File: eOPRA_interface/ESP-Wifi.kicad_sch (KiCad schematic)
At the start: 18 parts, among them SW1 SW_Push

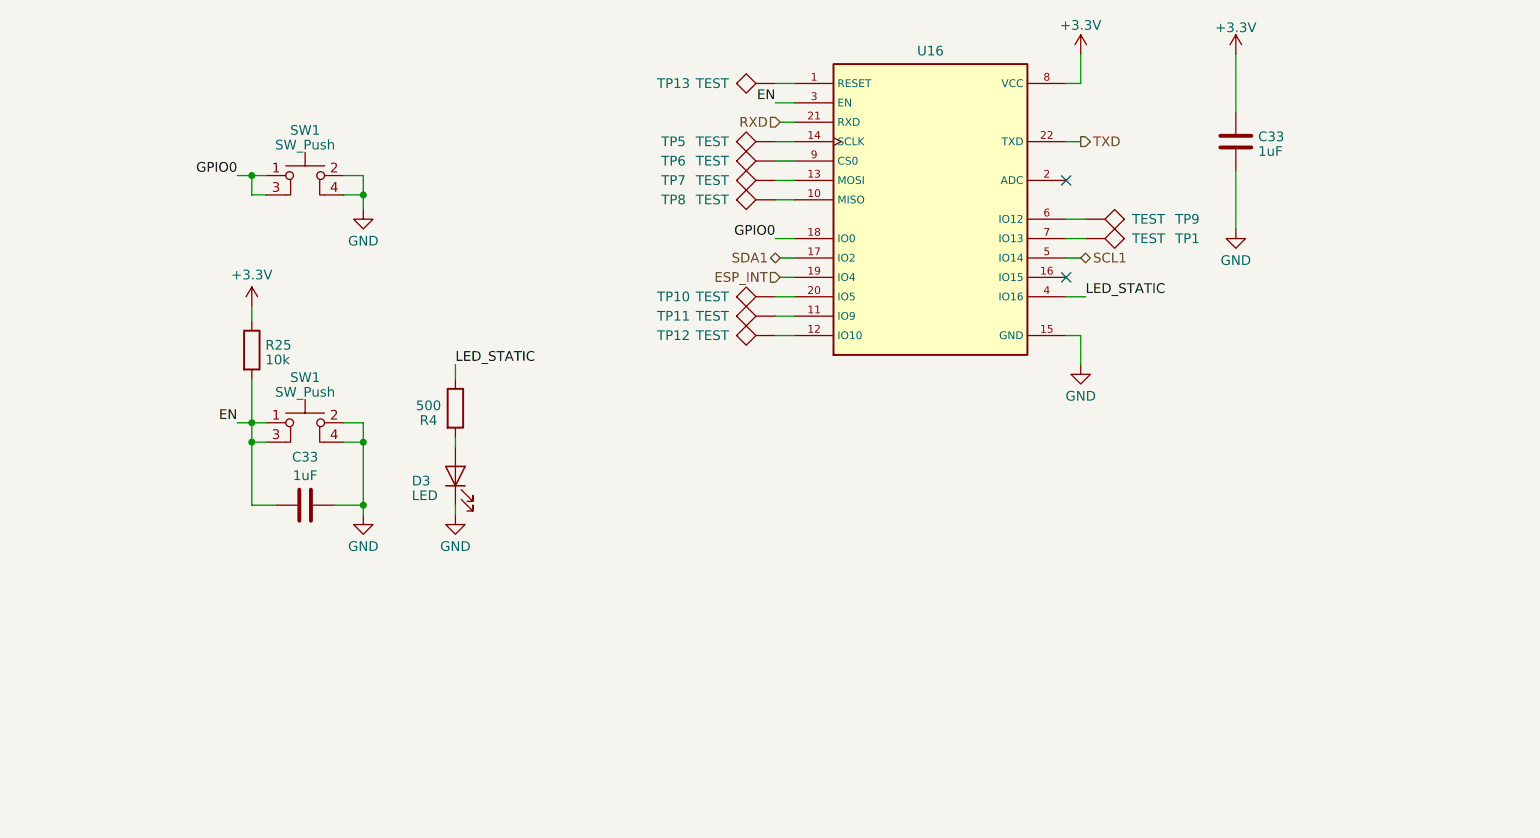
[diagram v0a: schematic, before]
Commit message: stuff
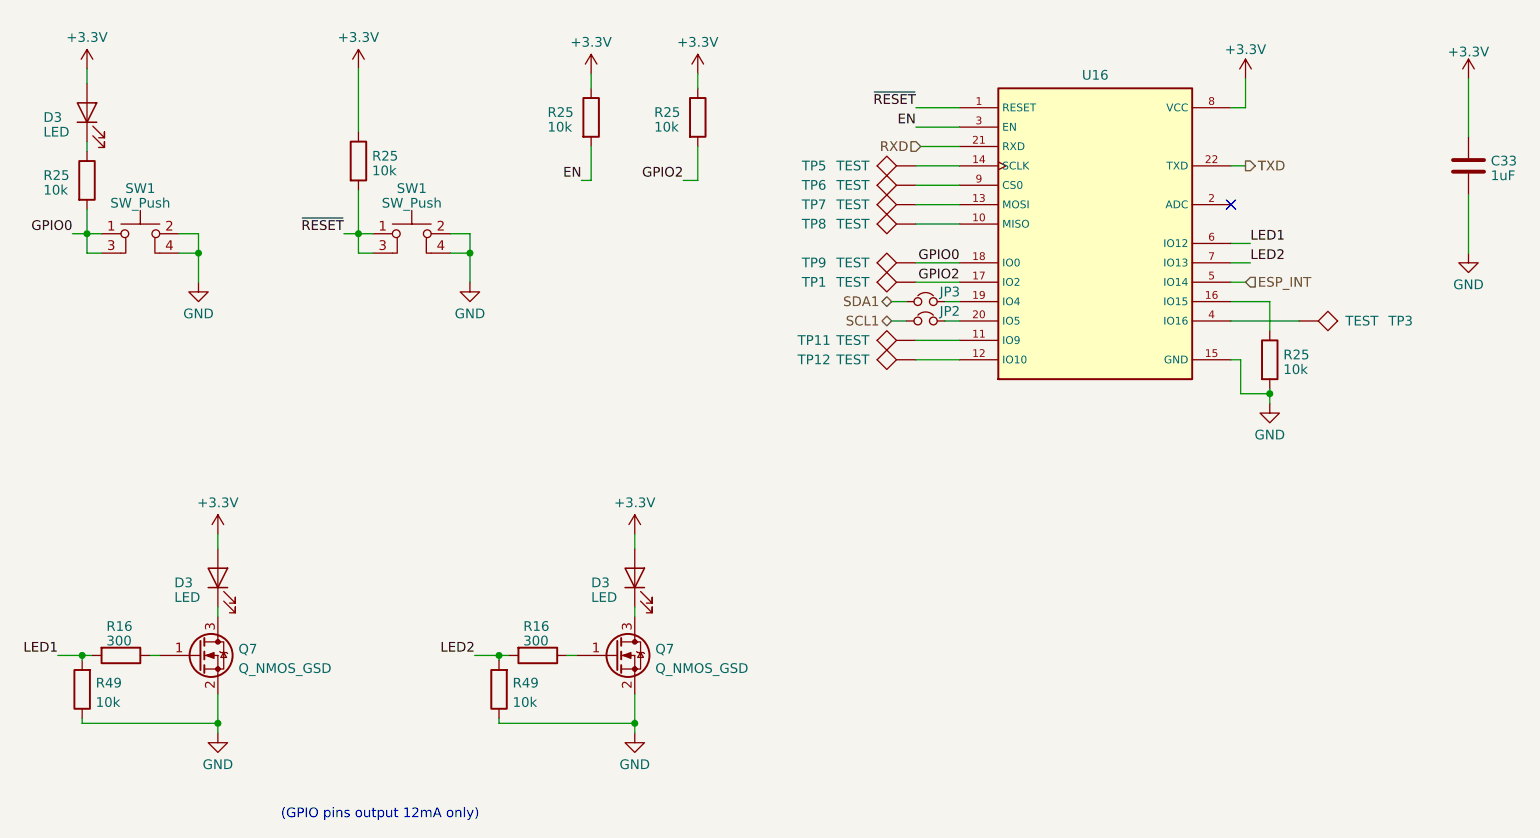
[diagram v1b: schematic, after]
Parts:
- removed C33: 1uF, 2_Passives_Resistors_SMD_IPC:R_1005_402_A, symbol 2.passive:C
- removed D3: LED, 1_Semi_Discrete_Diodes_SMD:D_0603, symbol 1.semi.opto:LED
- removed R4: 500, 2_Passives_Resistors_SMD_IPC:R_1608_603_B, symbol 2.passive:R
- removed TP10, TP13: TEST, 0_misc:test_point_1.0mm_square, symbol 5.connector.interconnect:TEST
- added D3 (x3): LED, 1_Semi_Discrete_Diodes_SMD:D_0603, symbol 1.semi.opto:LED
- added JP2, JP3: ~, 0_misc:SolderJumper-2_P1.3mm_Bridged_RoundedPad1.0x1.5mm, symbol 2.passive:Jumper_NC_Small
- added Q7 (x2): Q_NMOS_GSD, 1_Semi_TO_SOT:SOT-323FL, symbol 1.semi.discrete:Q_NMOS_GSD
- added R16 (x2): 300, 2_Passives_Resistors_SMD_IPC:R_1608_603_B, symbol 2.passive:R
- added R25 (x4), R49 (x2): 10k, 2_Passives_Resistors_SMD_IPC:R_1608_603_B, symbol 2.passive:R
- added TP3: TEST, 0_misc:test_point_1.0mm_square, symbol 5.connector.interconnect:TEST
- C33: footprint 2_Passives_Resistors_SMD_IPC:R_1005_402_A -> 2_Passives_Capacitors_SMD_IPC:C_1005_402_A; PN (none) -> 2,2
- R25: PN (none) -> 1,2
- SW1: PN (none) -> 9,4
- U16: PN (none) -> 5,4
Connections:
- net +3V3: now also D3.2 (A), D3.2 (A), D3.2 (A), R25.1, R25.1
- net EN: now also R25.2; no longer R25.2, SW1.1, SW1.3
- net ESP_INT: now also U16.5 (IO14); no longer U16.19 (IO4)
- net GND: now also Q7.2 (S), Q7.2 (S), R25.2, R49.1, R49.1
- net GPIO0: now also TP9.1, R25.2
- net SCL1: now also JP2.1; no longer U16.5 (IO14)
- net SDA1: now also JP3.1; no longer U16.17 (IO2)
- net ~{RESET}: now reaches U16.1 (RESET)
- net ~{RESET}: now also R25.2, SW1.1, SW1.3
- net GPIO2: now reaches TP1.1
- net GPIO2: now also U16.17 (IO2), R25.2; no longer U16.7 (IO13)
- net at U16.16 (IO15): now also R25.1
- net at U16.20 (IO5): now also JP2.2
- net LED1: now reaches U16.6 (IO12)
- net LED1: now also R16.2, R49.2; no longer TP9.1
- net LED_STATIC: no longer names the net of U16.4 (IO16)
- net LED_STATIC: now also TP3.1
- new net: D3.1 (K), Q7.3 (D) (x2)
- new net: D3.1 (K), R25.1
- new net: Q7.1 (G), R16.1 (x2)
- new net: JP3.2, U16.19 (IO4)
- new net LED2: R16.2, R49.2, U16.7 (IO13)
- no-connect marks 2 -> 1
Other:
- note added: "(GPIO pins output 12mA only)"
- moved on the sheet: C33, R25, SW1, TP11, TP12, TP5, TP6, TP7, TP8, U16

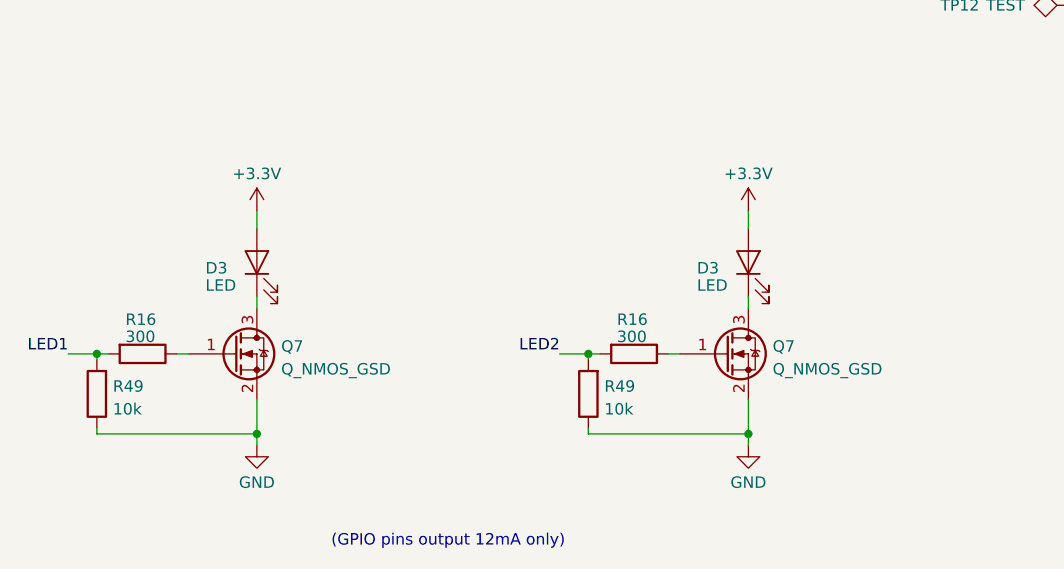
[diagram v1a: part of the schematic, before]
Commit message: stuff
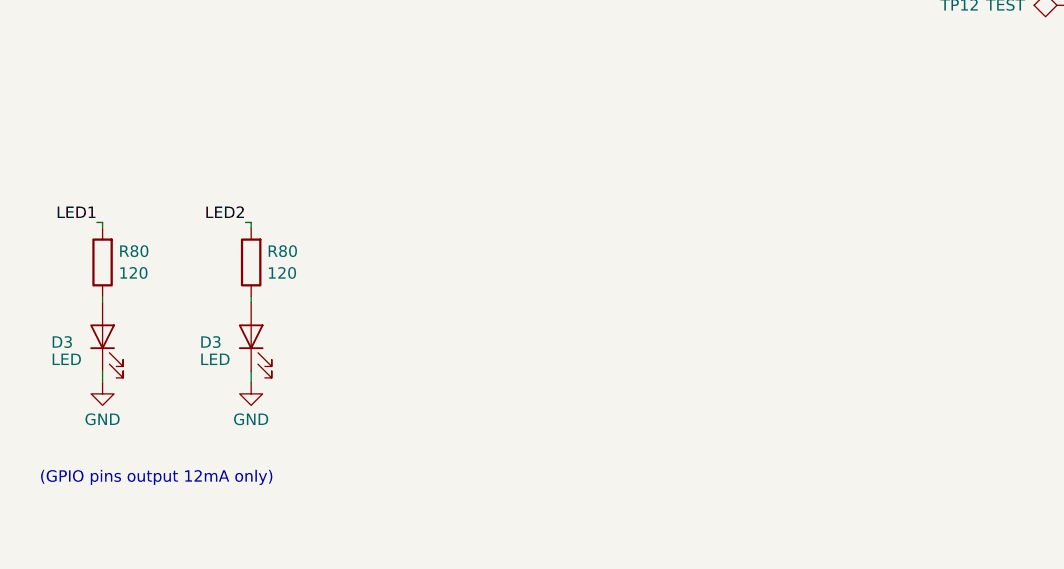
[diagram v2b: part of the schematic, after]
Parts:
- removed Q7 (x2): Q_NMOS_GSD, 1_Semi_TO_SOT:SOT-323FL, symbol 1.semi.discrete:Q_NMOS_GSD
- removed R16 (x2): 300, 2_Passives_Resistors_SMD_IPC:R_1608_603_B, symbol 2.passive:R
- removed R49 (x2): 10k, 2_Passives_Resistors_SMD_IPC:R_1608_603_B, symbol 2.passive:R
- added R80 (x2): 120, 2_Passives_Resistors_SMD_IPC:R_1005_402_A, symbol 2.passive:R
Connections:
- net +3V3: no longer D3.2 (A), D3.2 (A)
- net GND: now also D3.1 (K), D3.1 (K)
- net LED1: now also R80.2
- net LED2: now also R80.2
- new net: D3.2 (A), R80.1 (x2)
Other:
- moved on the sheet: D3
